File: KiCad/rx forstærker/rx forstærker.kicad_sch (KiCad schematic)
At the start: 11 parts, among them U1 MCP6002-xMC

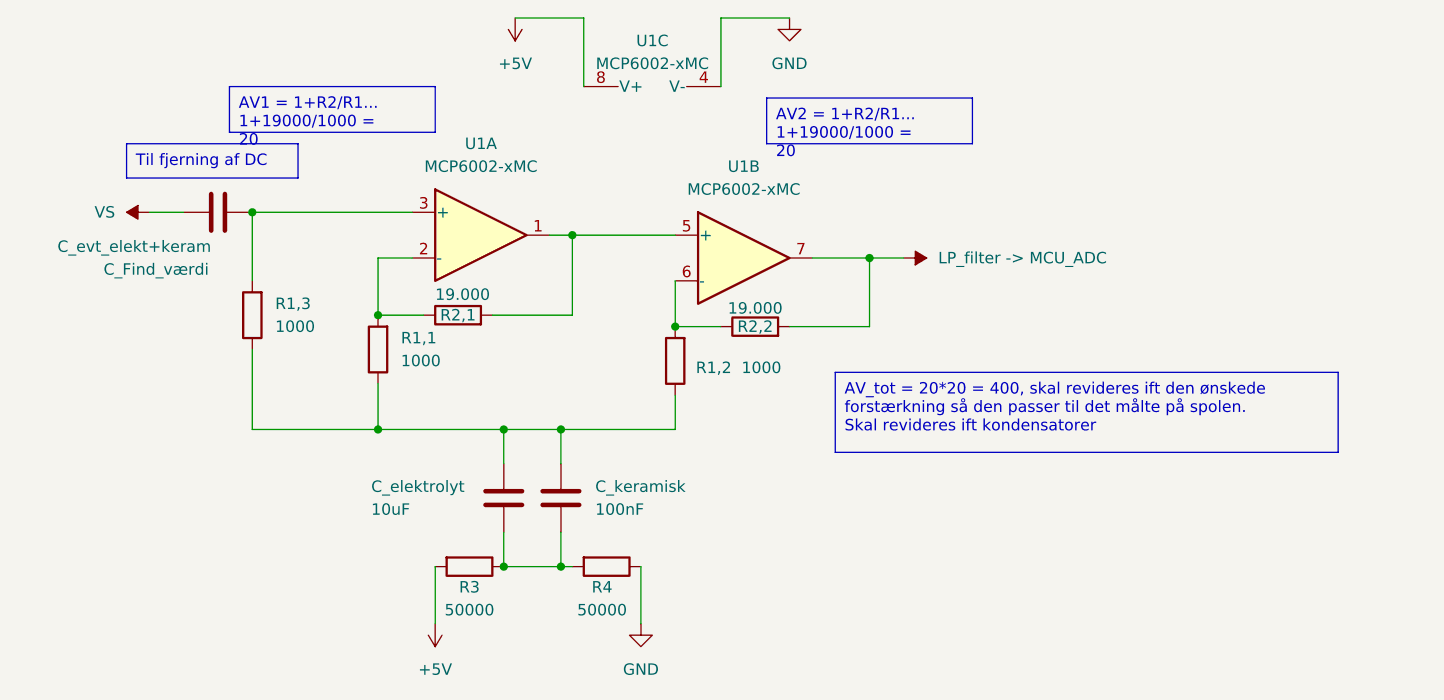
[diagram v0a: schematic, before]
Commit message: Rx forstærker uden kond
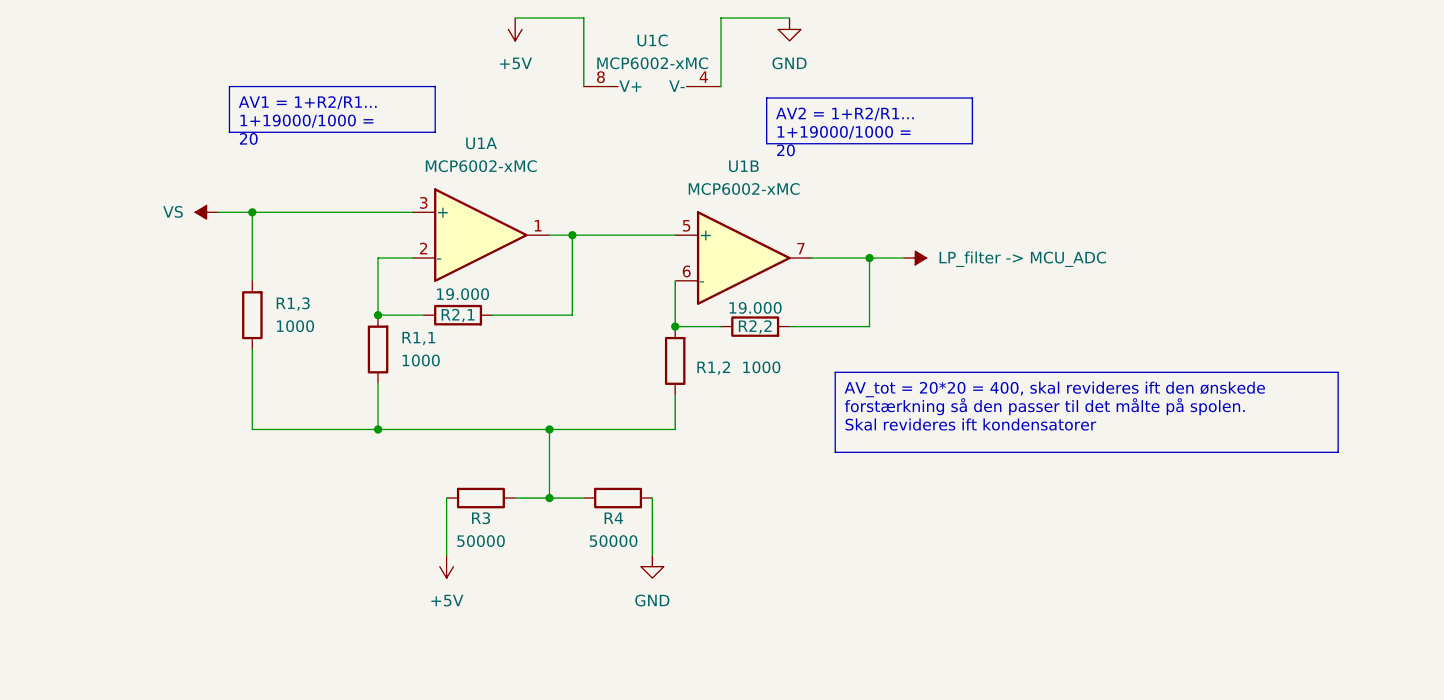
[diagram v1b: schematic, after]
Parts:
- removed C_elektrolyt: 10uF, symbol Device:C
- removed C_evt_elekt+keram: C_Find_værdi, symbol Device:C
- removed C_keramisk: 100nF, symbol Device:C
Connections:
- net VS: now also R1,3.2, U1.3 (+)
- net at R1,1.1, R1,2.1, R1,3.1: now also R3.1, R4.2
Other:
- moved on the sheet: R3, R4
